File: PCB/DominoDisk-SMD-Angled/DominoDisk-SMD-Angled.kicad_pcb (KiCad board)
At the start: 4 copper layers, 45 x 35.2 mm, 29 parts, among them J1 Daisy port out, J2 ICSP_ISP6, J3 Daisy port in, J4 UART, K1 TF-104 MicroSD card holder, U1 PC817C-S, U2 ATmega328P-AU, U3 TXB0104PWR level shifter, U4 SE5218ALG voltage regulator, Y1 CSTNE16M0V530000R0 Resonator

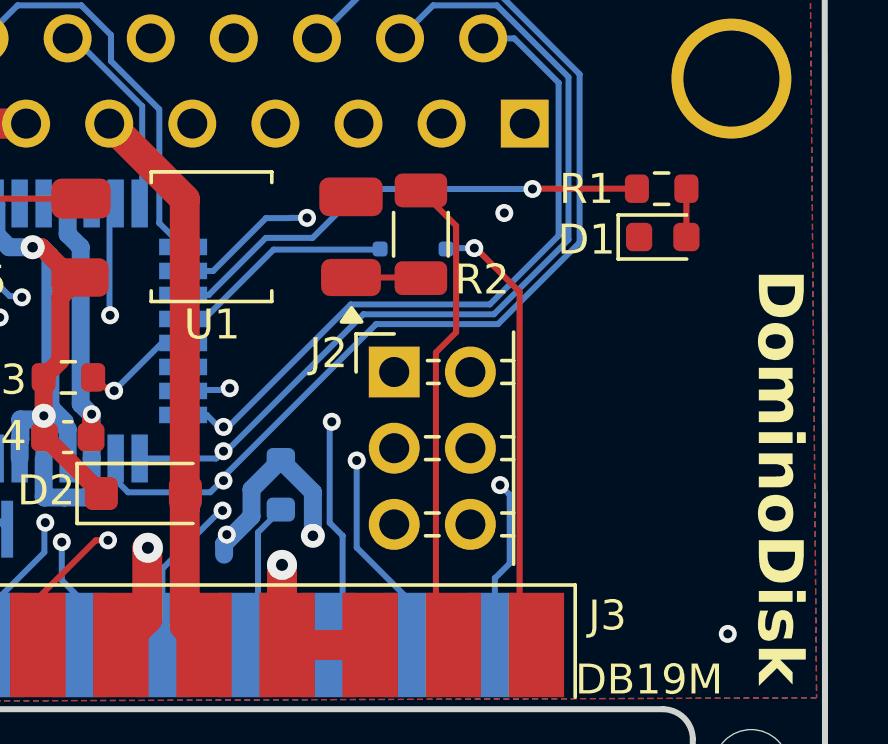
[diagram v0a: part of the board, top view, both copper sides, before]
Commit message: Angled version
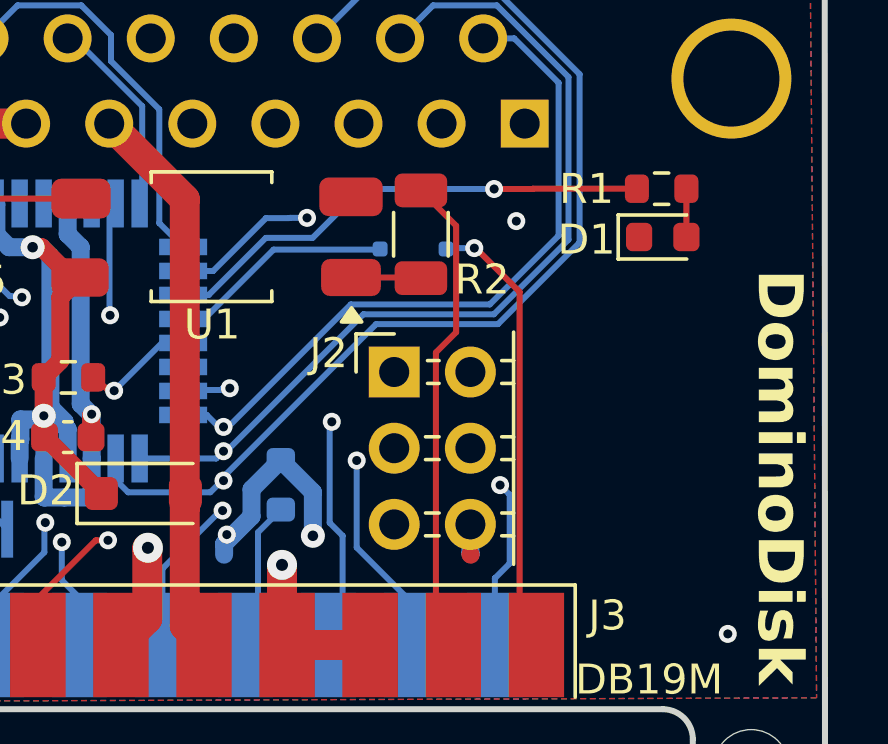
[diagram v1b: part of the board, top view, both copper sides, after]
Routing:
- net GND: track 44.2 -> 45.2 mm
